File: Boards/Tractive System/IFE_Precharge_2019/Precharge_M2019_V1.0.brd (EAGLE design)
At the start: 39.4 x 45.7 mm, 21 parts

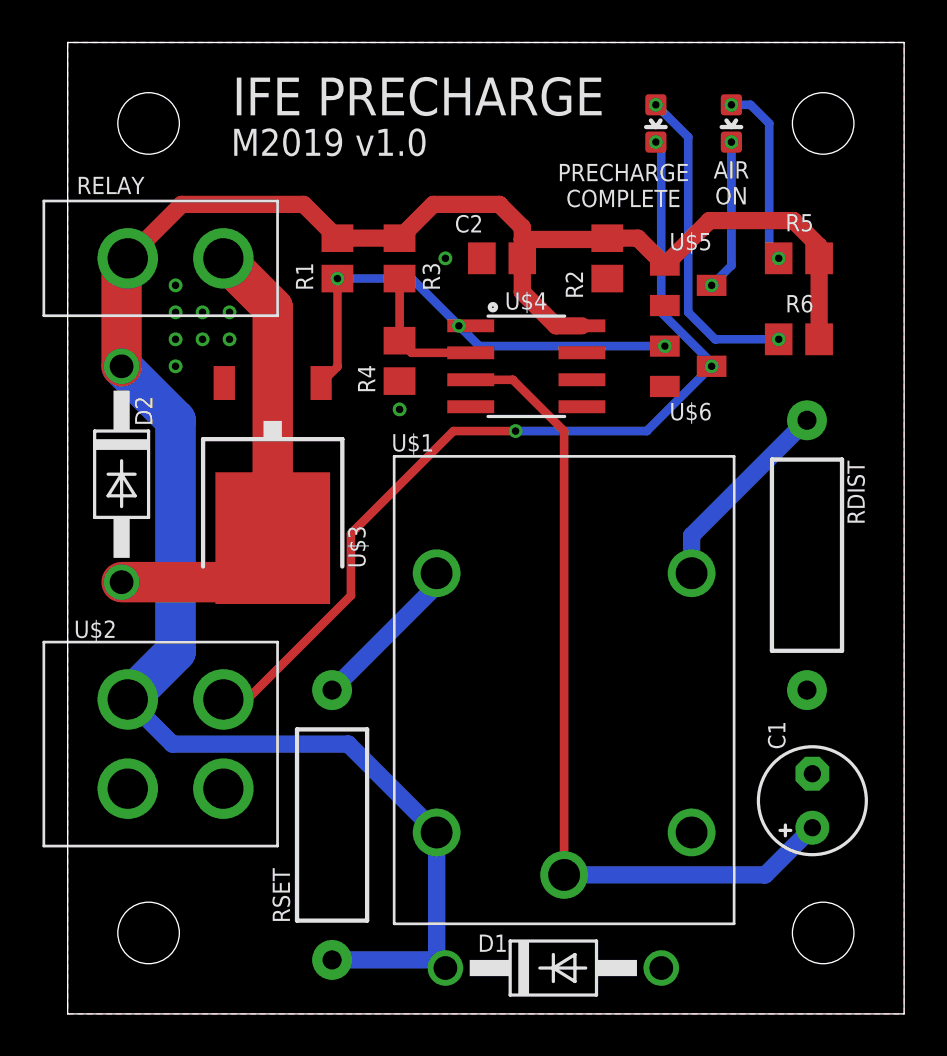
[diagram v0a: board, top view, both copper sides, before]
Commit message: More precharge organization
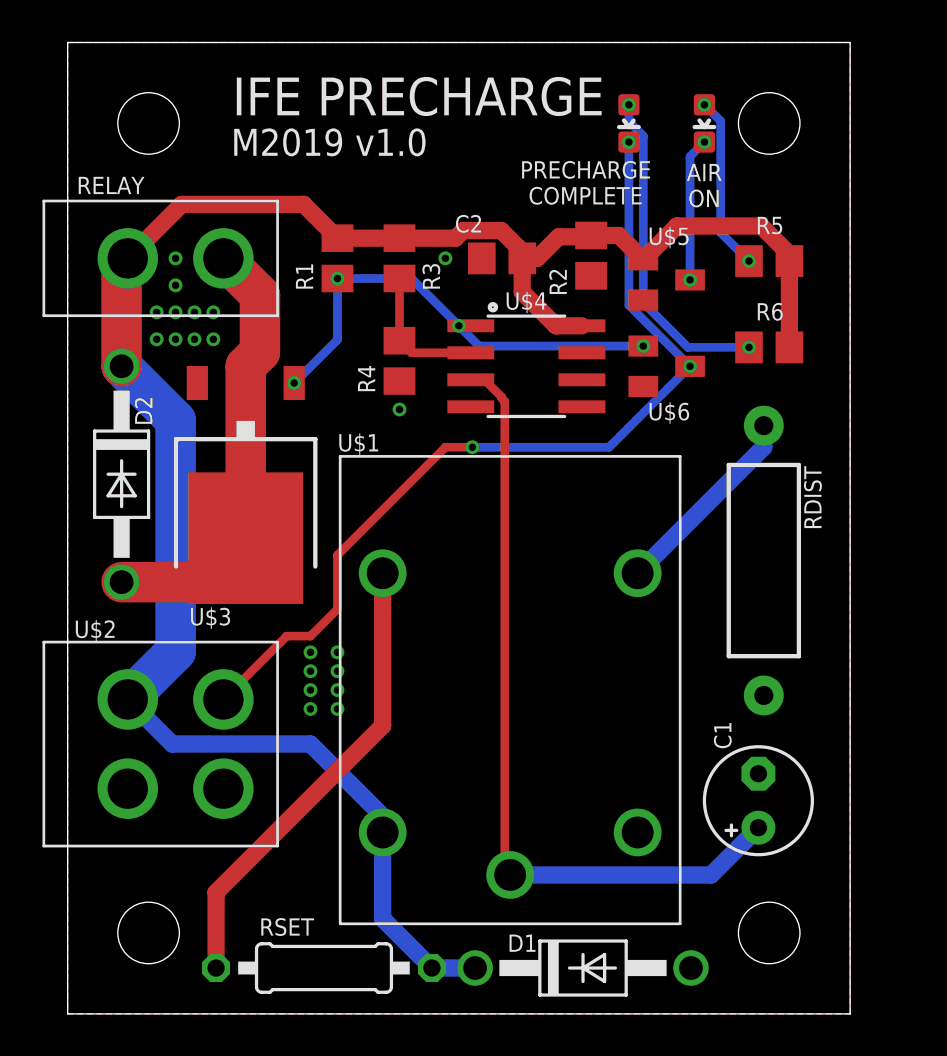
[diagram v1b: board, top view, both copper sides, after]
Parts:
- RSET: value 350k -> 220k; device SparkFun-Resistors:AXIAL-0.5 -> rcl:0207/10
- moved RSET 6.74 mm to (12.1, 2.16), turned to 0 degrees
- moved C1 2.54 mm to (32.5, 10.0)
- moved U$1 2.54 mm to (20.8, 15.2)
- moved RDIST 2.05 mm to (32.8, 21.3)
- moved R6 1.45 mm to (33.0, 31.4)
- moved R5 1.40 mm to (33.0, 35.4)
- moved D1 1.40 mm to (24.3, 2.16)
- moved AIR_ON 1.27 mm to (30.0, 41.9)
- moved PRECHARGE 1.27 mm to (26.4, 41.9)
- moved U$3 1.27 mm to (8.38, 24.9)
- moved U$5 1.05 mm to (28.2, 34.5)
- moved U$6 1.02 mm to (28.2, 30.5)
- moved R2 0.77 mm to (24.6, 35.7)
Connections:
- net N$1: now also RSET.1; no longer RSET.P$1
- net V+: now also RSET.2; no longer RSET.P$2
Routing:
- net N$1: track 7.54 -> 21.8 mm
- net V+: track 100.2 -> 92.6 mm
- net N$2: track 38.9 -> 37.1 mm
- net PRECHARGE_COMPLETE: track 42.8 -> 41.7 mm
- net N$4: track 22.1 -> 21.4 mm
- net PRECHARGE: track 22.5 -> 22.0 mm, vias 3 -> 4
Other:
- board size 39.4 x 45.7 mm -> 36.8 x 45.7 mm
